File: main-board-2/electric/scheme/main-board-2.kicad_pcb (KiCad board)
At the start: 2 copper layers, 85 x 56 mm, 124 parts, among them K1 power-switch, K2 usb-power-switch, P1 batt, P10 rst, P11 screw-1, P13 screw-2, P14 gpio-big, P15 gpio-small, P16 moto-1, P17 moto-2, P3 trigger-btn, P4 CONN_3X2, P5 reg-short-to-gnd-1, P6 reg-short-to-gnd-2, P7 bootloader, P8 cross board conn, P9 rst, Q1 IRLML2244, Q10 IRLML2244, Q11 sot223, Q12 bc857, Q13 irlml2244, Q2 BC847, Q3 IRLML2244, Q4 IRLML2244, Q5 BC847, Q6 BC847, Q7 BC847, Q8 BC847, Q9 IRLML2244, U1 LM317AEMP, U2 LM317AT, U3 LM317AEMP, U4 LM317AT, U5 LM293, U6 L298, U7 MINI-USB-B, X1 8MHz

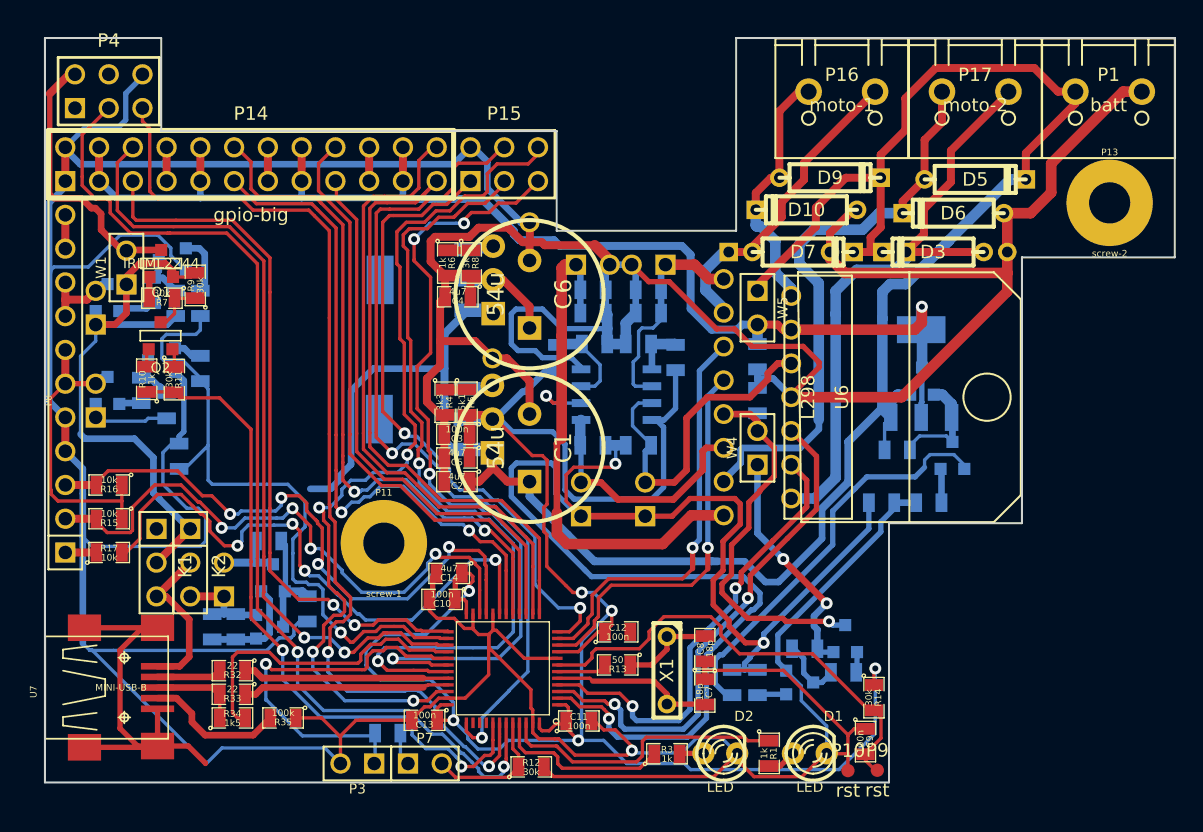
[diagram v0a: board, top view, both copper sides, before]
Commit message: Routing...
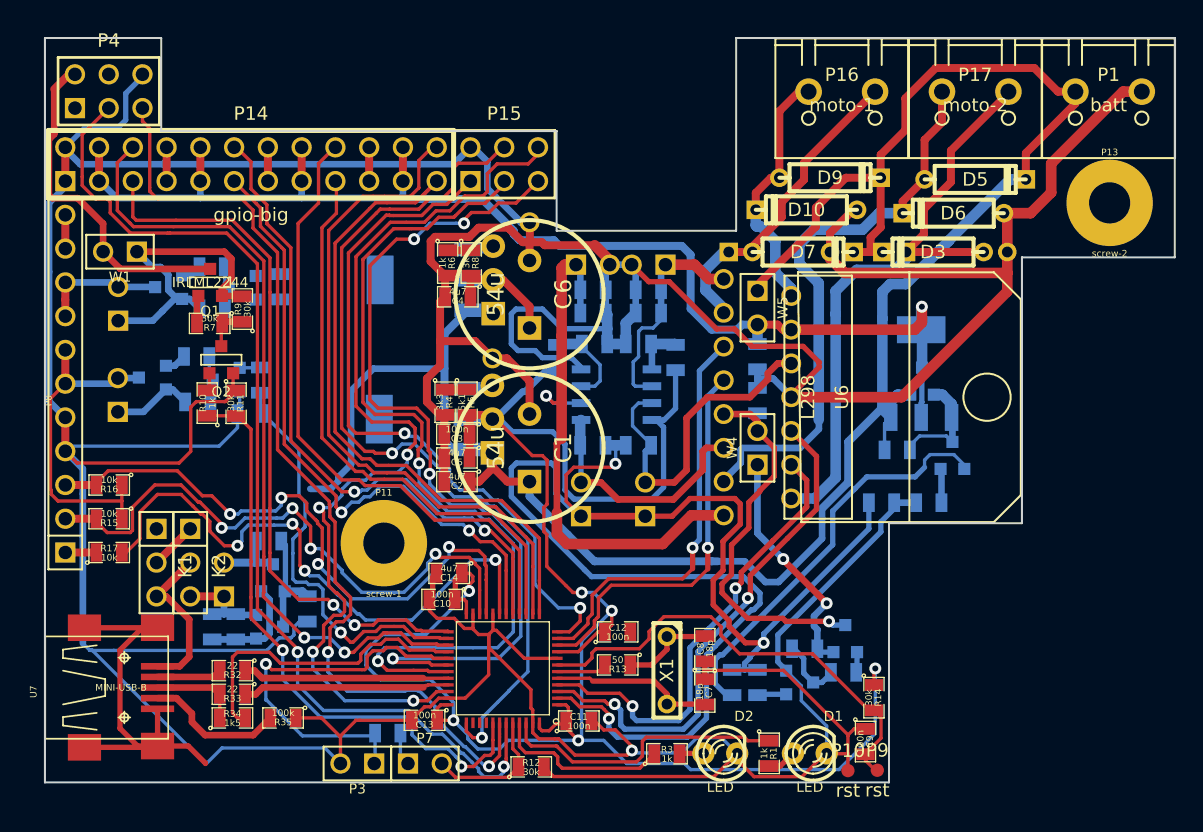
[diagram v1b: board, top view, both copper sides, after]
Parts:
- moved R24 6.24 mm to (158.9, 153.3), turned to 0 degrees
- moved R22 6.10 mm to (161.2, 143.7)
- moved Q5 5.66 mm to (158.3, 143.8)
- moved Q6 5.08 mm to (157.1, 150.7)
- moved R11 4.98 mm to (157.9, 152.5)
- moved Q2 4.91 mm to (156.8, 149.2)
- moved R10 4.90 mm to (155.7, 152.5)
- moved R18 4.89 mm to (156.1, 142.2), turned to 180 degrees
- moved R19 4.89 mm to (154.9, 149.0), turned to 180 degrees
- moved Q3 4.66 mm to (152.8, 143.7), turned to 90 degrees
- moved R23 4.59 mm to (159.7, 150.7)
- moved R7 4.06 mm to (155.9, 146.5)
- moved R9 3.96 mm to (158.4, 145.4)
- moved Q1 3.95 mm to (155.9, 143.4)
- moved Q4 3.51 mm to (151.6, 150.5), turned to 90 degrees
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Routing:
- net /addon-pwr-en: track 49.9 -> 31.4 mm
- net /+5V: track 62.0 -> 52.6 mm
- net /rpi-pwr-en: track 50.7 -> 45.4 mm
- net /rx: track 61.5 -> 66.4 mm
- net /swd-io: track 66.6 -> 71.5 mm
- net GND: track 523.1 -> 518.6 mm
- net N-0000062: track 4.51 -> 0.00 mm
- net /gpio-9: track 48.7 -> 53.2 mm
- net /tx: track 61.5 -> 65.9 mm
- net /gpio-8: track 47.8 -> 51.3 mm
- net /swd-clk: track 63.5 -> 66.8 mm
- net /addon-5V: track 6.20 -> 9.44 mm
- net /gpio-4: track 47.4 -> 50.4 mm
- net N-000003: track 23.0 -> 25.8 mm
- net /gpio-7: track 45.1 -> 47.9 mm
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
